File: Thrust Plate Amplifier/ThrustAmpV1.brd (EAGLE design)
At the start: 104.9 x 77.5 mm, 87 parts, among them U1 INA126PA, U2 INA126PA, U3 INA126PA, U4 INA126PA, U5 LP2985AIM5-3.3, U6 LP2985AIM5-5.0/NOPB

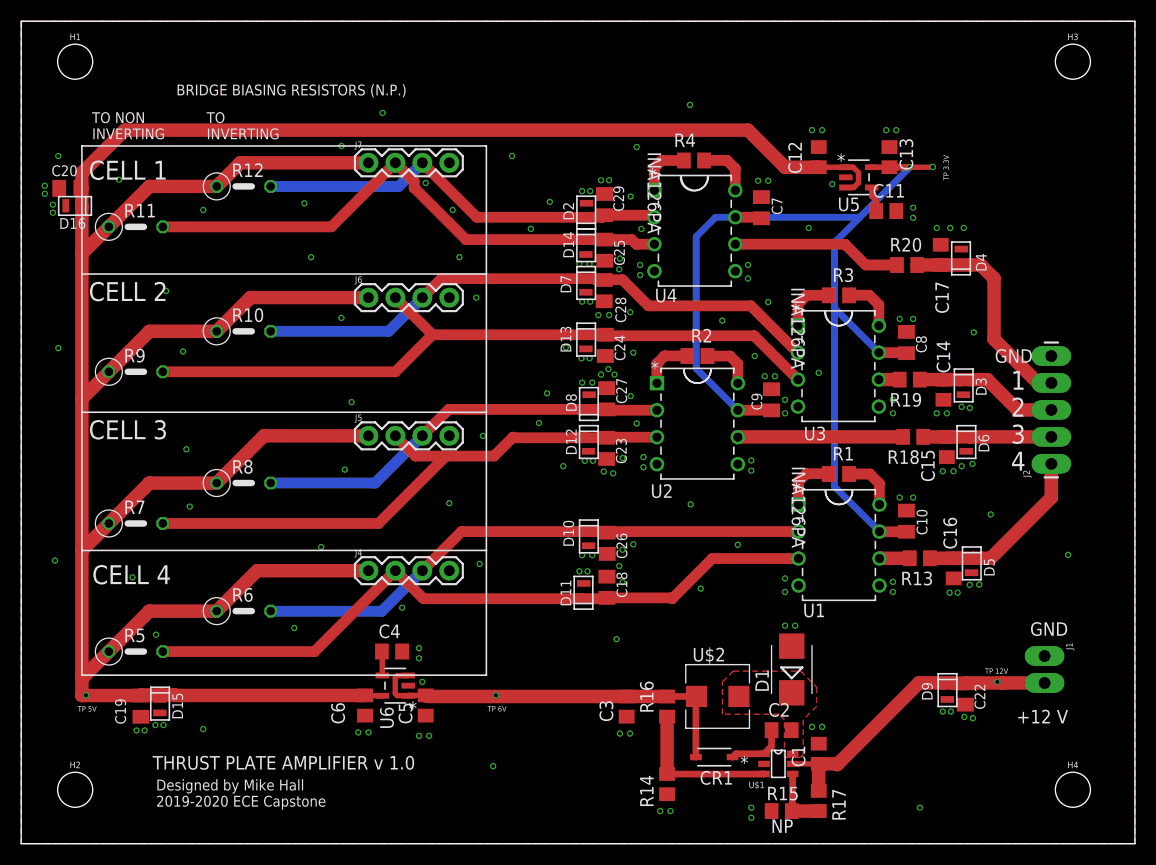
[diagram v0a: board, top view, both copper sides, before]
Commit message: Minor Plate Amp changes
Un-derping
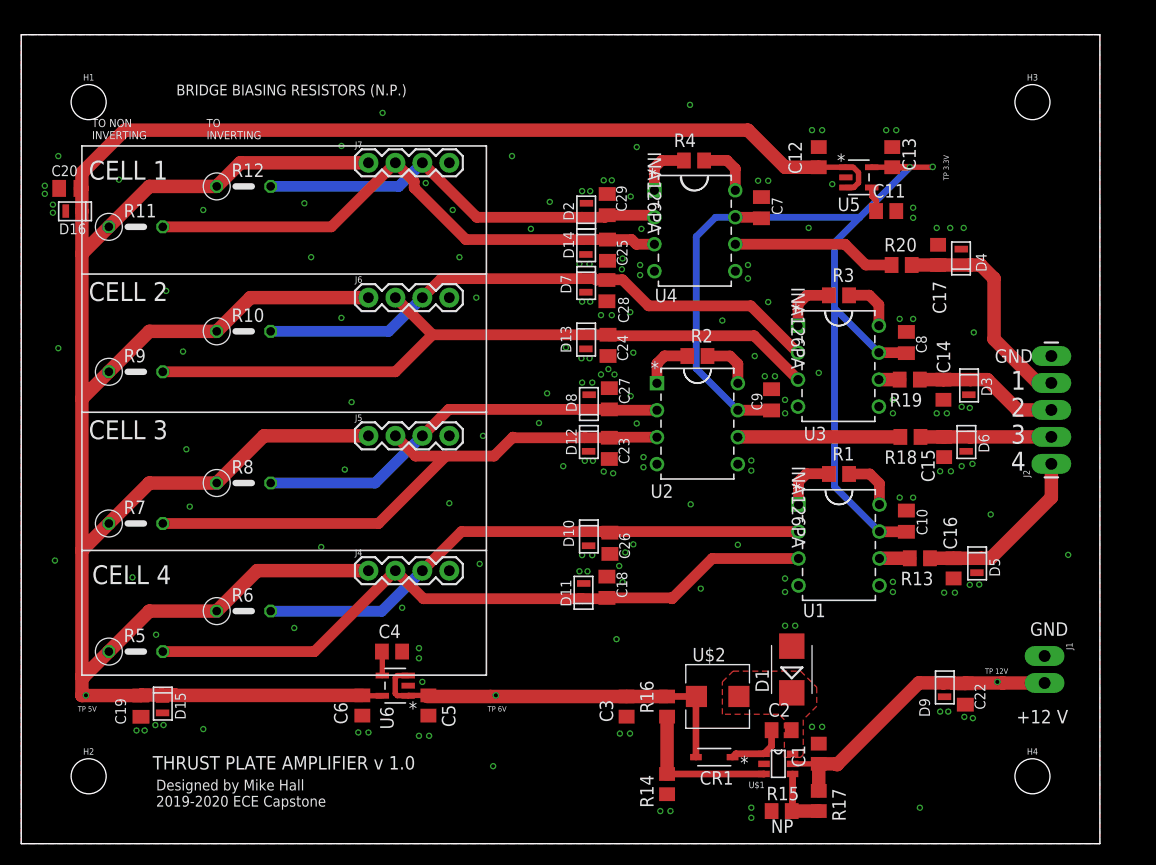
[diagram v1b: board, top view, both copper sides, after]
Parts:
- R17: value 500 k -> 499 k
- moved H3 5.39 mm to (95.2, 69.8)
- moved H1 4.02 mm to (6.35, 69.8)
- moved H4 4.02 mm to (95.2, 6.35)
- moved H2 1.80 mm to (6.35, 6.35)
- moved D16 0.51 mm to (4.83, 59.7)
- moved D3 0.51 mm to (89.2, 42.9)
- moved D5 0.51 mm to (89.9, 26.2)
- moved R20 0.51 mm to (82.9, 54.5)
- moved D9 0.36 mm to (86.9, 14.5)
- moved C13 0.25 mm to (82.0, 64.7)
- moved C15 0.25 mm to (86.9, 37.4)
- moved C17 0.25 mm to (86.4, 55.5)
- moved C24 0.25 mm to (55.3, 46.9)
- moved C29 0.25 mm to (55.2, 60.2)
- moved D15 0.25 mm to (13.2, 13.0)
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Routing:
- net 12V: track 30.8 -> 30.2 mm
- net N$17: track 16.0 -> 15.5 mm
- net N$23: track 14.3 -> 13.8 mm
- net N$24: track 21.5 -> 22.1 mm
- net N$19: track 17.9 -> 17.4 mm
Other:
- board size 104.9 x 77.5 mm -> 101.6 x 76.2 mm
